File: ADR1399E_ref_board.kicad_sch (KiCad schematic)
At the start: 32 parts, among them J1 USB_C_Receptacle_PowerOnly_6P, J2 Conn_01x02_Pin, U1 ADR1399KEZ, U2 LT3042xMSE, U3 TPS61085DGK, U4 TL331, U5 OPA182IDR

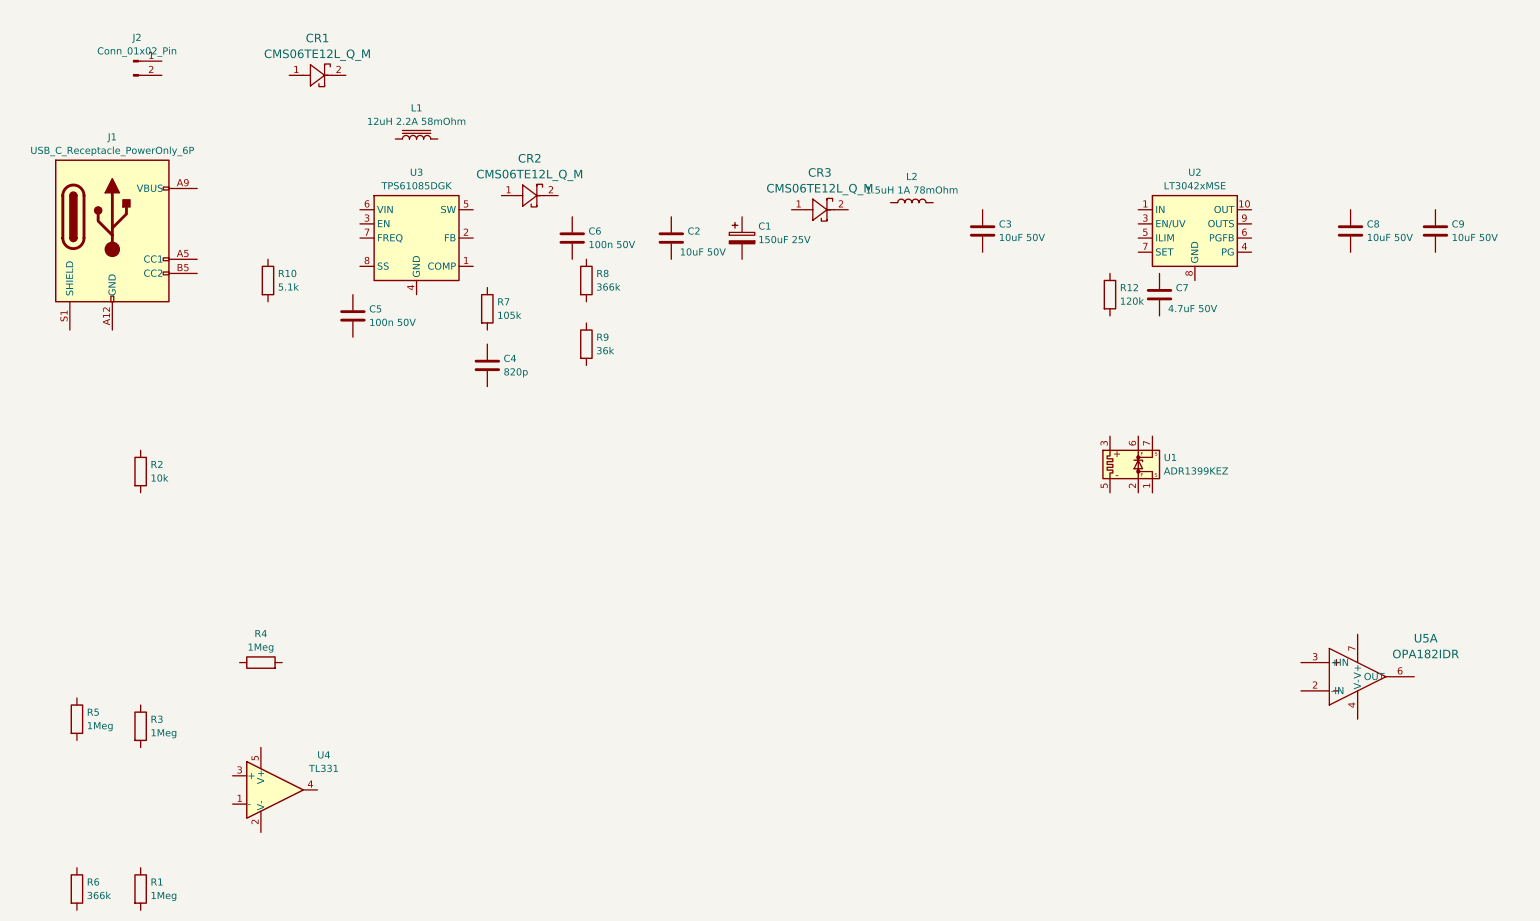
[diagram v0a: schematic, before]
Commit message: moving forward
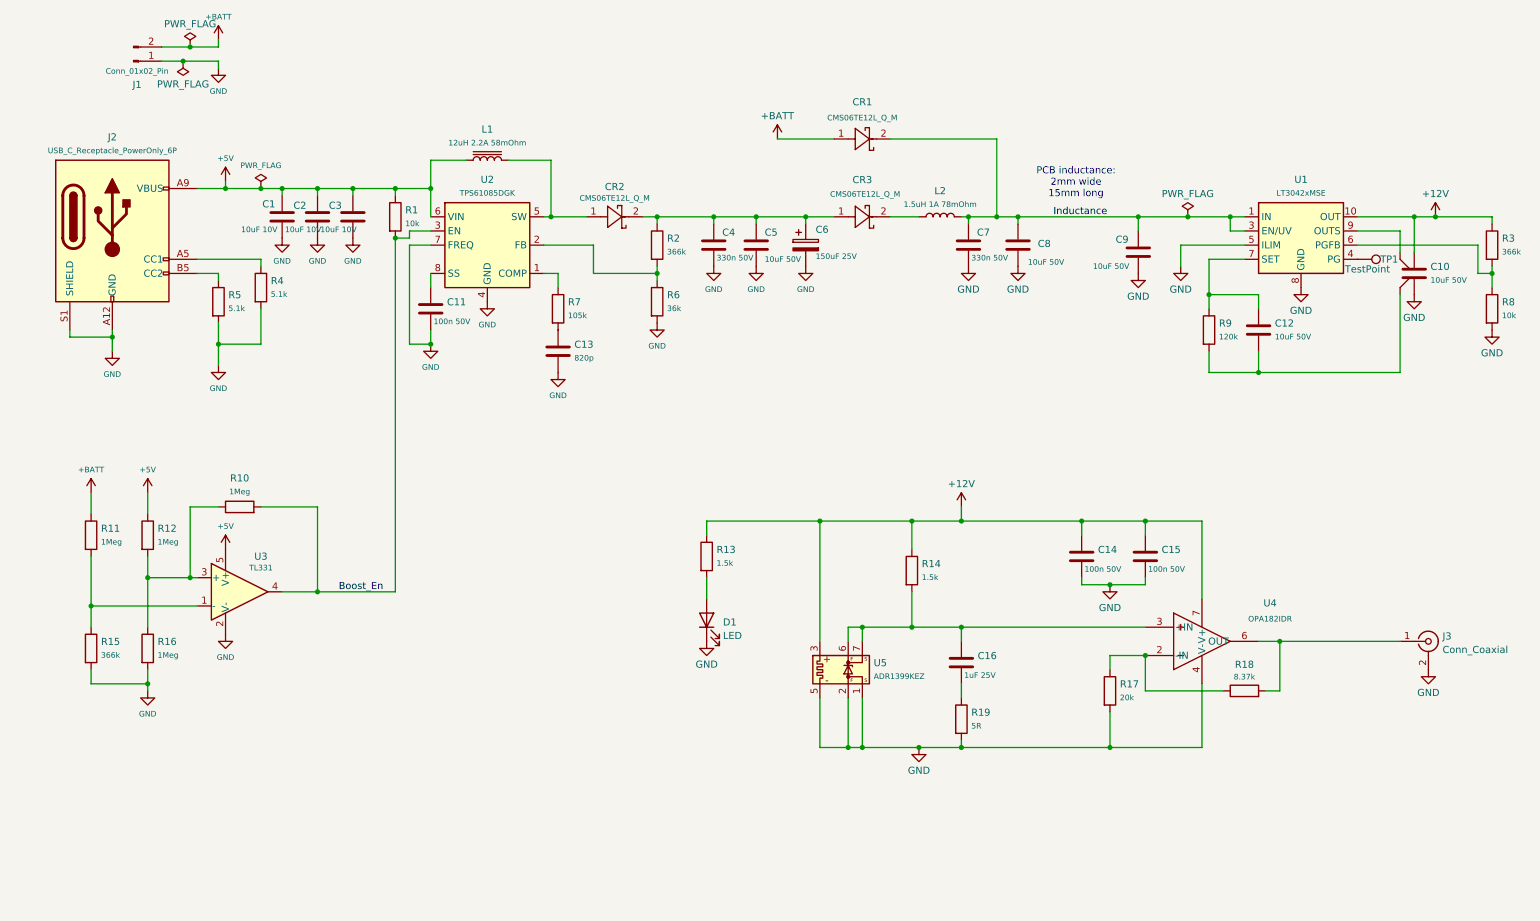
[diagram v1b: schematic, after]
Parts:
- removed C6: 100n 50V, Capacitor_SMD:C_0504_1310Metric_Pad0.83x1.28mm_HandSolder, symbol Device:C
- removed C8: 10uF 50V, Capacitor_SMD:C_1210_3225Metric_Pad1.33x2.70mm_HandSolder, symbol Device:C
- added C1, C2, C3: 10uF 10V, Capacitor_SMD:C_0805_2012Metric_Pad1.18x1.45mm_HandSolder, symbol Device:C
- added C10: 10uF 50V, nightmechanic_pcb:3225_Kelvin_4port, symbol nightmechanic_lib:Kelvin_Cap
- added C12: 10uF 50V, Capacitor_SMD:C_1210_3225Metric_Pad1.33x2.70mm_HandSolder, symbol Device:C
- added C14, C15: 100n 50V, Capacitor_SMD:C_0603_1608Metric_Pad1.08x0.95mm_HandSolder, symbol Device:C
- added C16: 1uF 25V, Capacitor_SMD:C_0603_1608Metric_Pad1.08x0.95mm_HandSolder, symbol Device:C
- added C4: 330n 50V, Capacitor_SMD:C_0603_1608Metric_Pad1.08x0.95mm_HandSolder, symbol Device:C
- added D1: LED, LED_SMD:LED_1206_3216Metric_Pad1.42x1.75mm_HandSolder, symbol Device:LED
- added J3: Conn_Coaxial, Connector_Coaxial:SMA_Molex_73251-1153_EdgeMount_Horizontal, symbol Connector:Conn_Coaxial
- added R13, R14: 1.5k, Resistor_SMD:R_0805_2012Metric_Pad1.20x1.40mm_HandSolder, symbol Device:R
- added R17: 20k, Resistor_SMD:R_0805_2012Metric_Pad1.20x1.40mm_HandSolder, symbol Device:R
- added R18: 8.37k, Resistor_SMD:R_0805_2012Metric_Pad1.20x1.40mm_HandSolder, symbol Device:R
- added R19: 5R, Resistor_SMD:R_0805_2012Metric_Pad1.20x1.40mm_HandSolder, symbol Device:R
- added R3: 366k, Resistor_SMD:R_0805_2012Metric_Pad1.20x1.40mm_HandSolder, symbol Device:R
- added R5: 5.1k, Resistor_SMD:R_0805_2012Metric_Pad1.20x1.40mm_HandSolder, symbol Device:R
- added R8: 10k, Resistor_SMD:R_0805_2012Metric_Pad1.20x1.40mm_HandSolder, symbol Device:R
- added TP1: TestPoint, TestPoint:TestPoint_Pad_D1.5mm, symbol Connector:TestPoint
- C11: renamed from C5; footprint Capacitor_SMD:C_0504_1310Metric_Pad0.83x1.28mm_HandSolder -> Capacitor_SMD:C_0603_1608Metric_Pad1.08x0.95mm_HandSolder
- C13: renamed from C4; footprint Capacitor_SMD:C_0504_1310Metric_Pad0.83x1.28mm_HandSolder -> Capacitor_SMD:C_0603_1608Metric_Pad1.08x0.95mm_HandSolder
- C7: value 4.7uF 50V -> 330n 50V; footprint Capacitor_SMD:C_1206_3216Metric_Pad1.33x1.80mm_HandSolder -> Capacitor_SMD:C_0603_1608Metric_Pad1.08x0.95mm_HandSolder
- renumbered C2 to C5, C1 to C6, C3 to C8, J2 to J1, J1 to J2, R2 to R1, R4 to R10, R5 to R11, R3 to R12, R6 to R15, R1 to R16, R8 to R2, R10 to R4, R9 to R6, R12 to R9, U2 to U1, U3 to U2, U4 to U3, U5 to U4, U1 to U5
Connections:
- net at R15.1: now also R11.2, U3.1 (-)
- net GND: now reaches R15.2
- net GND: now also C11.2, C13.2, C5.2, C6.2, C7.2, C8.2, C9.2, J1.1 (Pin_1), J2.A12 (GND), J2.B12 (GND), J2.S1 (SHIELD), R16.2, R4.2, R6.2, U1.11 (GND), U1.5 (ILIM), U1.8 (GND), U2.4 (GND), U2.7 (FREQ), U3.2 (V-), U4.4 (V-), U5.1 (-REFS), U5.2 (-REFF), U5.5 (HEATER-), C1.2, C10.2, C14.2, C15.2, C2.2, C3.2, C4.2, D1.1 (K), J3.2 (Ext), R17.2, R19.2, R5.2, R8.2
- net +12V: now reaches U5.3 (HEATER+)
- net +12V: now also U1.10 (OUT), U4.7 (V+), C10.3, C14.1, C15.1, R13.1, R14.1, R3.1
- net at U5.6 (+REFF): now also U4.3 (+IN), U5.7 (+REFS), C16.1, R14.2
- net +BATT: now reaches R11.1
- net +BATT: now also CR1.1, J1.2 (Pin_2)
- net at R7.1: now also U2.1 (COMP)
- net at R7.2: now also C13.1
- net Inductance: now reaches CR1.2
- net Inductance: now also C7.1, C8.1, C9.1, L2.2, U1.1 (IN), U1.2 (IN), U1.3 (EN/UV)
- net at U2.2 (FB): now also R2.2, R6.1
- net Boost_En: now reaches U2.3 (EN)
- net Boost_En: now also R1.2, R10.2, U3.4
- net at U2.5 (SW): now also CR2.1, L1.2
- net +5V: now reaches U2.6 (VIN)
- net +5V: now also J2.A9 (VBUS), J2.B9 (VBUS), L1.1, R1.1, R12.1, U3.5 (V+), C1.1, C2.1, C3.1
- net at U2.8 (SS): now also C11.1
- net at C6.1: now also C5.1, CR2.2, CR3.1, R2.1, C4.1
- net at R4.1: now also J2.A5 (CC1)
- net at J2.B5 (CC2): now also R5.1
- net at U1.4 (PG): now also TP1.1
- net at U1.6 (PGFB): now also R3.2, R8.1
- net at U1.7 (SET): now also R9.1, C12.1
- net at U1.9 (OUTS): now also C10.4
- net at R12.2: now also R10.1, R16.1, U3.3 (+)
- net at L2.1: now also CR3.2
- net at R9.2: now also C10.1, C12.2
- net at U4.2 (-IN): now also R17.1, R18.1
- net at U4.6 (OUT): now also J3.1 (In), R18.2
- new net: D1.2 (A), R13.2
- new net: C16.2, R19.1
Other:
- note added: "PCB inductance: 2mm wide 15mm long"
- moved on the sheet: C11, C13, C5, C6, C8, C9, CR1, CR2, CR3, J1, L1, L2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
